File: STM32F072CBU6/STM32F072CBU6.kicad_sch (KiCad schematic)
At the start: 12 parts

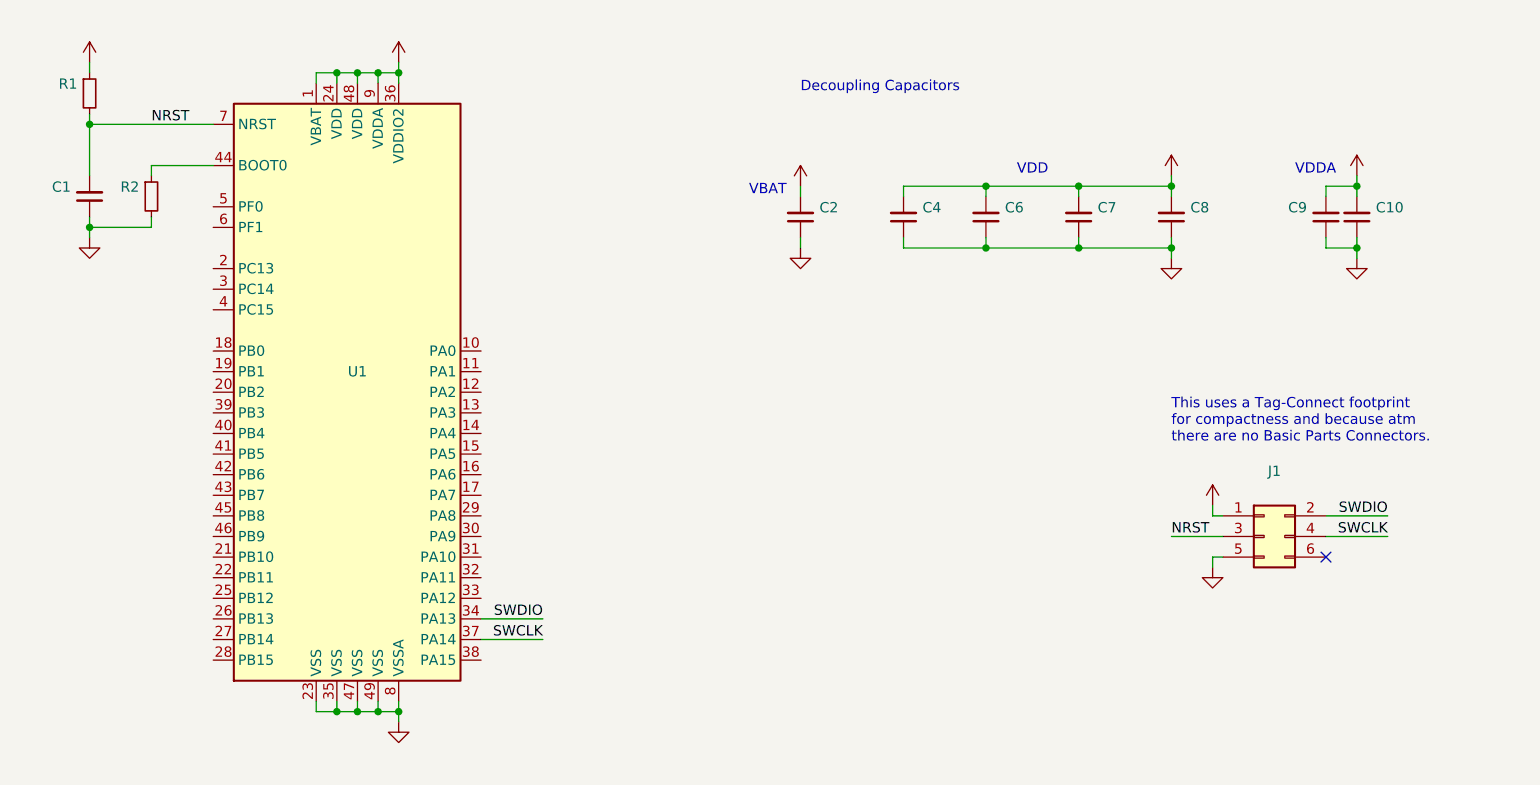
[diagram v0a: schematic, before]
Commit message: Reapply "Update modules to kicad v7 format"
This reverts commit fa5cc85431189ac7a3beedf0871b5723203ae43f.
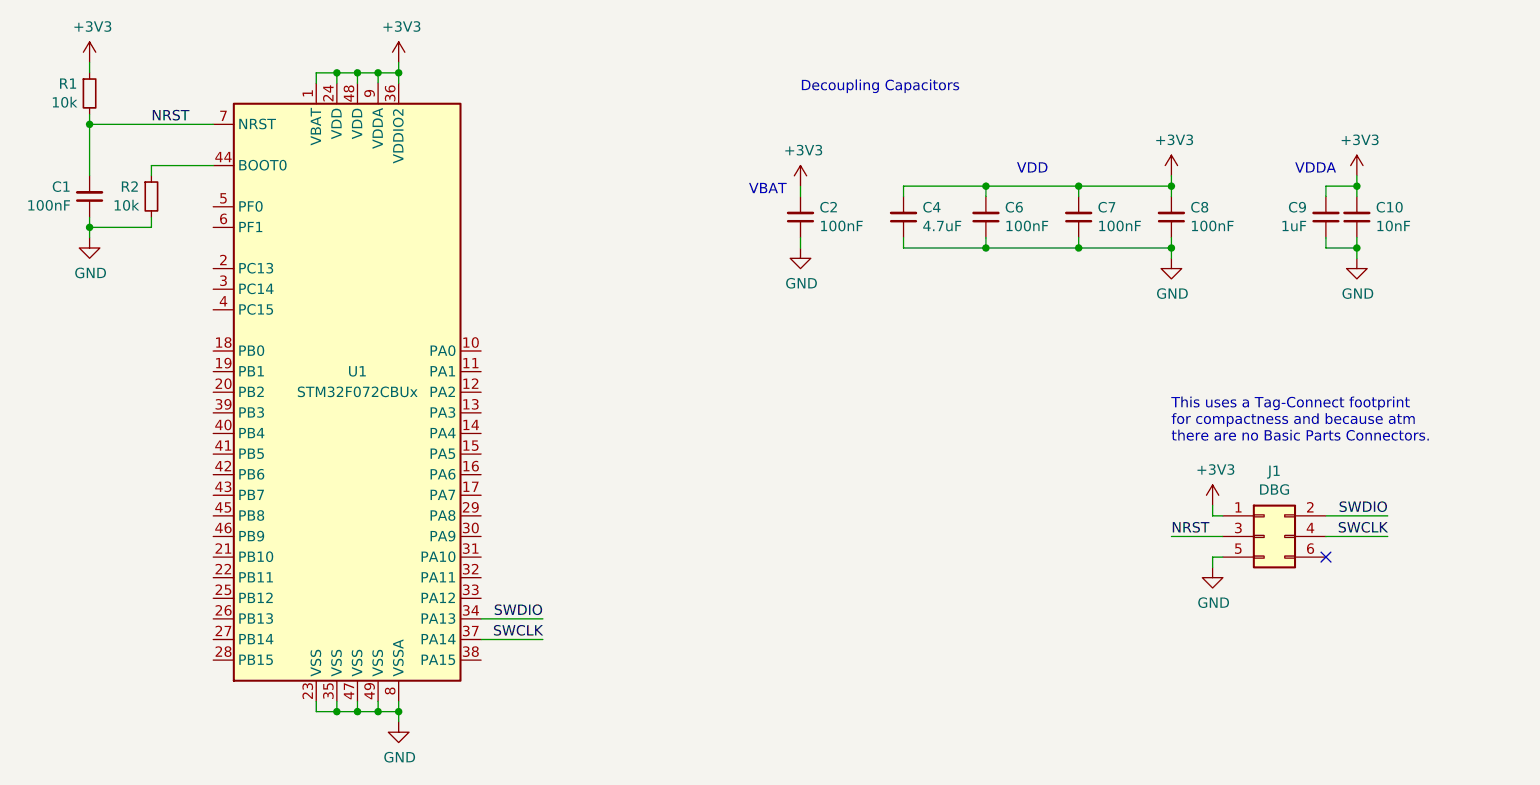
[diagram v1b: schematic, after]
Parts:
- C1, C2, C6, C7, C8: value (none) -> 100nF; footprint (none) -> Capacitor_SMD:C_0402_1005Metric
- C10: value (none) -> 10nF; footprint (none) -> Capacitor_SMD:C_0402_1005Metric
- C4: value (none) -> 4.7uF; footprint (none) -> Capacitor_SMD:C_0402_1005Metric
- C9: value (none) -> 1uF; footprint (none) -> Capacitor_SMD:C_0402_1005Metric
- J1: value (none) -> DBG; footprint (none) -> Connector:Tag-Connect_TC2030-IDC-NL_2x03_P1.27mm_Vertical
- R1, R2: value (none) -> 10k; footprint (none) -> Resistor_SMD:R_0402_1005Metric
- U1: value (none) -> STM32F072CBUx; footprint (none) -> Package_DFN_QFN:QFN-48-1EP_7x7mm_P0.5mm_EP5.6x5.6mm

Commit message: Revert "Update modules to kicad v7 format"
This reverts commit 3325eb02d48d3d222bc7f8945228a1814ae85736.
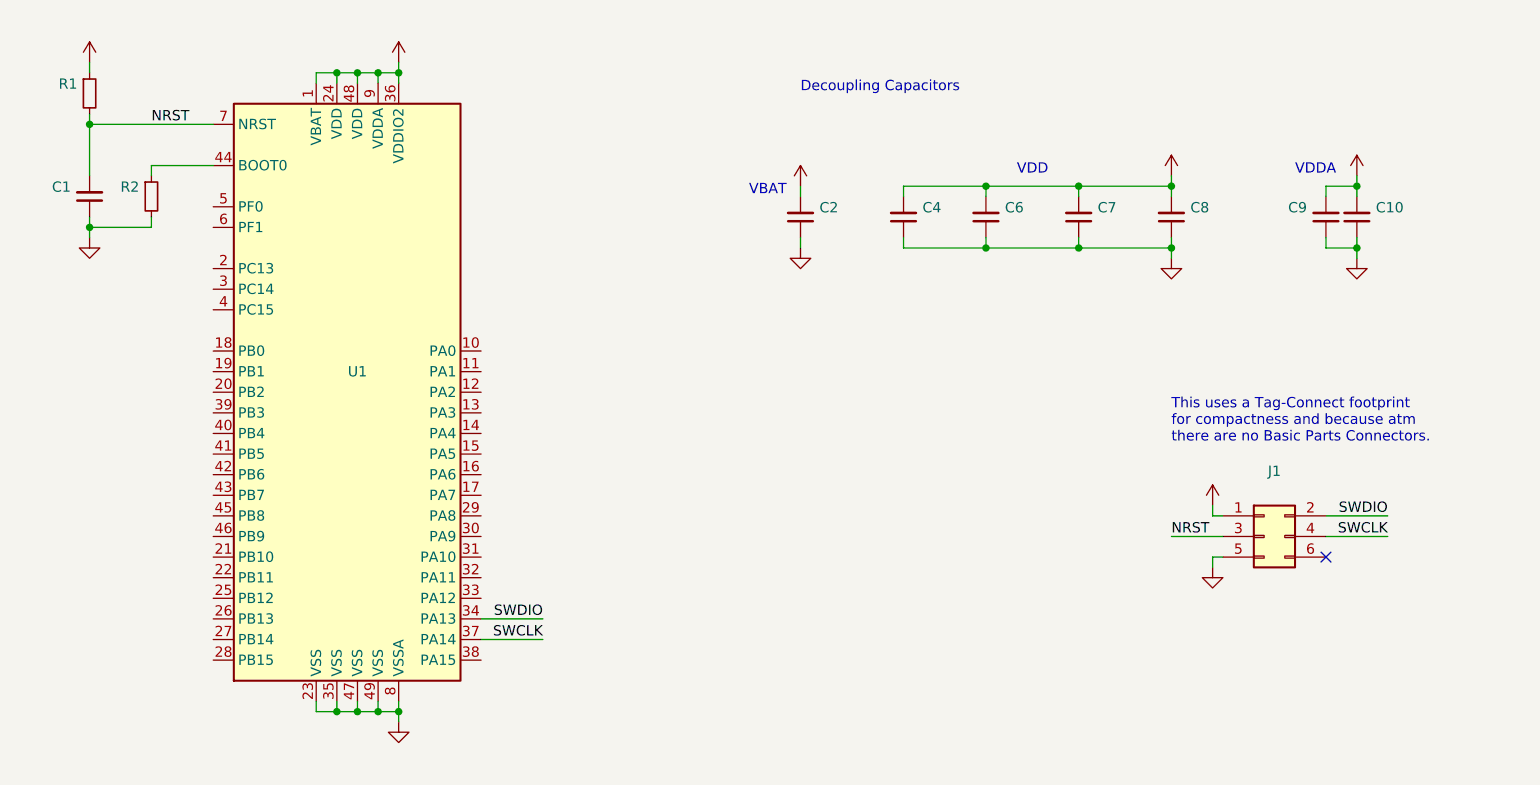
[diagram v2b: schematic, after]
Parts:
- C1, C2, C6, C7, C8: value 100nF -> (none); footprint Capacitor_SMD:C_0402_1005Metric -> (none)
- C10: value 10nF -> (none); footprint Capacitor_SMD:C_0402_1005Metric -> (none)
- C4: value 4.7uF -> (none); footprint Capacitor_SMD:C_0402_1005Metric -> (none)
- C9: value 1uF -> (none); footprint Capacitor_SMD:C_0402_1005Metric -> (none)
- J1: value DBG -> (none); footprint Connector:Tag-Connect_TC2030-IDC-NL_2x03_P1.27mm_Vertical -> (none)
- R1, R2: value 10k -> (none); footprint Resistor_SMD:R_0402_1005Metric -> (none)
- U1: value STM32F072CBUx -> (none); footprint Package_DFN_QFN:QFN-48-1EP_7x7mm_P0.5mm_EP5.6x5.6mm -> (none)
